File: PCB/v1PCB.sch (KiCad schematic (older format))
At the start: 223 parts, among them SW1 SW_PUSH, SW2 SW_PUSH, U1 STM32F072CBUx, U2 MCP1700-3302E_SOT23

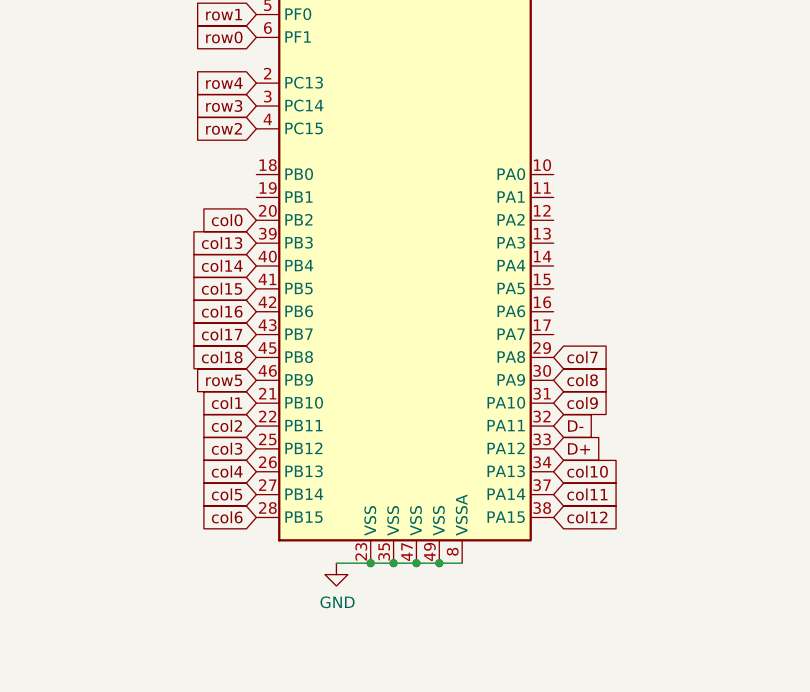
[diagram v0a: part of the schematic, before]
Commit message: Updates to CAD and PCB
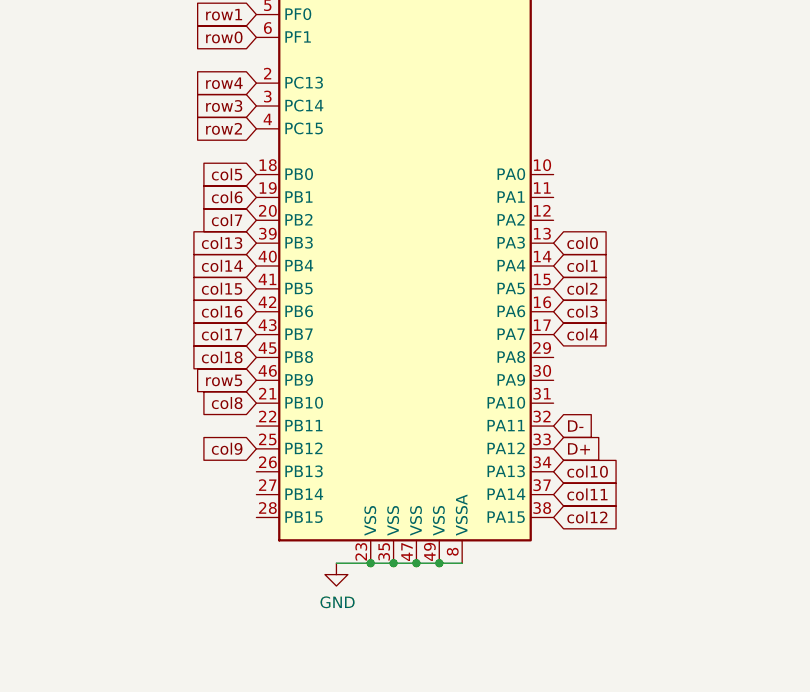
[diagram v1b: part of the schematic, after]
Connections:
- net col0: now also U1.13 (PA3); no longer U1.20 (PB2)
- net col1: now also U1.14 (PA4); no longer U1.21 (PB10)
- net col2: now also U1.15 (PA5); no longer U1.22 (PB11)
- net col3: now also U1.16 (PA6); no longer U1.25 (PB12)
- net col4: now also U1.17 (PA7); no longer U1.26 (PB13)
- net col5: now also U1.18 (PB0); no longer U1.27 (PB14)
- net col6: now also U1.19 (PB1); no longer U1.28 (PB15)
- net col7: now also U1.20 (PB2); no longer U1.29 (PA8)
- net col8: now also U1.21 (PB10); no longer U1.30 (PA9)
- net col9: now also U1.25 (PB12); no longer U1.31 (PA10)
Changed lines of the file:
@@
 	1    0    0    -1
 $EndComp
-Text GLabel 10500 3600 0    50   Input ~ 0
+Text GLabel 11800 3000 2    50   Input ~ 0
 col3
-Text GLabel 10500 3700 0    50   Input ~ 0
+Text GLabel 11800 3100 2    50   Input ~ 0
 col4
-Text GLabel 10500 3800 0    50   Input ~ 0
+Text GLabel 10500 2400 0    50   Input ~ 0
 col5
-Text GLabel 10500 3900 0    50   Input ~ 0
+Text GLabel 10500 2500 0    50   Input ~ 0
 col6
-Text GLabel 11800 3200 2    50   Input ~ 0
+Text GLabel 10500 2600 0    50   Input ~ 0
 col7
 Text GLabel 10500 2700 0    50   Input ~ 0
@@
 Text GLabel 10500 2900 0    50   Input ~ 0
 col15
-Text GLabel 10500 3500 0    50   Input ~ 0
+Text GLabel 11800 2900 2    50   Input ~ 0
 col2
 Connection ~ 11100 1100
@@
 	1    0    0    -1
 $EndComp
-Text GLabel 10500 2600 0    50   Input ~ 0
-col0
-Text GLabel 10500 3400 0    50   Input ~ 0
+Text GLabel 11800 2800 2    50   Input ~ 0
 col1
-Text GLabel 10500 3300 0    50   Input ~ 0
-row5
 Connection ~ 5200 2000
 Connection ~ 5950 2200
@@
 Text GLabel 11800 3800 2    50   Input ~ 0
 col11
-Text GLabel 11800 3300 2    50   Input ~ 0
+Text GLabel 10500 3400 0    50   Input ~ 0
 col8
 Text GLabel 11800 3900 2    50   Input ~ 0
@@
 Text GLabel 11800 3700 2    50   Input ~ 0
 col10
-Text GLabel 11800 3400 2    50   Input ~ 0
+Text GLabel 10500 3600 0    50   Input ~ 0
 col9
-Text GLabel 10500 1800 0    50   Input ~ 0
-row0
-Text GLabel 10500 1700 0    50   Input ~ 0
-row1
-Text GLabel 10500 2200 0    50   Input ~ 0
-row2
-Text GLabel 10500 2100 0    50   Input ~ 0
-row3
-Text GLabel 10500 2000 0    50   Input ~ 0
-row4
 Text GLabel 10500 3200 0    50   Input ~ 0
 col18
@@
 Text GLabel 11800 3500 2    50   Input ~ 0
 D-
+Text GLabel 11800 2700 2    50   Input ~ 0
+col0
+Text GLabel 10500 3300 0    50   Input ~ 0
+row5
+Text GLabel 10500 2000 0    50   Input ~ 0
+row4
+Text GLabel 10500 2100 0    50   Input ~ 0
+row3
+Text GLabel 10500 2200 0    50   Input ~ 0
+row2
+Text GLabel 10500 1700 0    50   Input ~ 0
+row1
+Text GLabel 10500 1800 0    50   Input ~ 0
+row0
 $EndSCHEMATC

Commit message: Nearing final production
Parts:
- F1: footprint Fuse:Fuse_1206_3216Metric -> Fuse:Fuse_0603_1608Metric
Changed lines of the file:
@@
 F 0 "F1" V 17055 3100 50  0000 C CNN
 F 1 "Polyfuse (1A)" V 16964 3100 50  0000 C CNN
-F 2 "Fuse:Fuse_1206_3216Metric" H 16900 2900 50  0001 L CNN
+F 2 "Fuse:Fuse_0603_1608Metric" H 16900 2900 50  0001 L CNN
 F 3 "~" H 16850 3100 50  0001 C CNN
 	1    16850 3100

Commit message: Updates
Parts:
- C1, C10, C2, C3, C4, C5, C6, C7, C8, C9: symbol Device:C_Small -> v1PCB-rescue:C_Small-Device
- D_0, D_1, D_10, D_100, D_11, D_12, D_13, D_14, D_15, D_16, D_17, D_18, D_19, D_2, D_20, D_21, D_22, D_23, D_24, D_25, D_26, D_27, D_28, D_29, D_3, D_30, D_31, D_32, D_33, D_34, D_35, D_36, D_37, D_38, D_39, D_4, D_40, D_41, D_42, D_43, D_44, D_45, D_46, D_47, D_48, D_49, D_5, D_50, D_51, D_52, D_53, D_54, D_55, D_56, D_57, D_58, D_59, D_6, D_60, D_61, D_62, D_63, D_64, D_65, D_66, D_67, D_68, D_69, D_7, D_70, D_71, D_72, D_73, D_74, D_75, D_76, D_77, D_78, D_79, D_8, D_80, D_81, D_82, D_83, D_84, D_85, D_86, D_87, D_88, D_89, D_9, D_90, D_91, D_92, D_93, D_94, D_95, D_96, D_97, D_98, D_99: symbol Device:D_Small -> v1PCB-rescue:D_Small-Device
- F1: symbol Device:Polyfuse_Small -> v1PCB-rescue:Polyfuse_Small-Device
- R1, R2, R3, R4, R5: symbol Device:R_Small -> v1PCB-rescue:R_Small-Device
- U1: symbol MCU_ST_STM32F0:STM32F072CBUx -> v1PCB-rescue:STM32F072CBUx-MCU_ST_STM32F0
- U2: symbol Regulator_Linear:MCP1700-3302E_SOT23 -> v1PCB-rescue:MCP1700-3302E_SOT23-Regulator_Linear
